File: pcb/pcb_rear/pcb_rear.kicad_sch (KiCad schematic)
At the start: 23 parts, among them J1 MicroLab Input, J2 Pump, J3 DFRobot O2, J4 DFRobot NH3, Q1 T2N7002AK, Q2 T2N7002AK, Q3 T2N7002AK, Q4 T2N7002AK, U1 USEQGSE CO2, U2 USEQGSE CH4, U3 XC9265A331MR-G, U4 XC9265A331MR-G

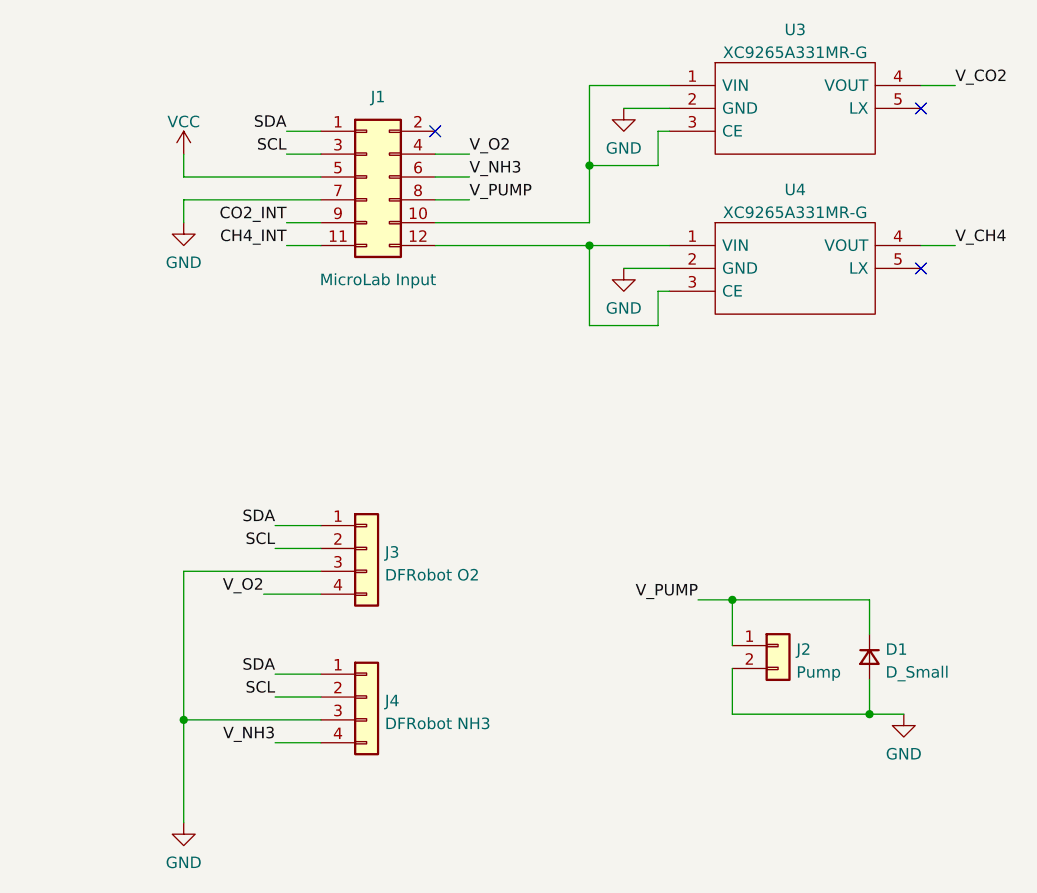
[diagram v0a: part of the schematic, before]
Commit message: front pcb 1st rev
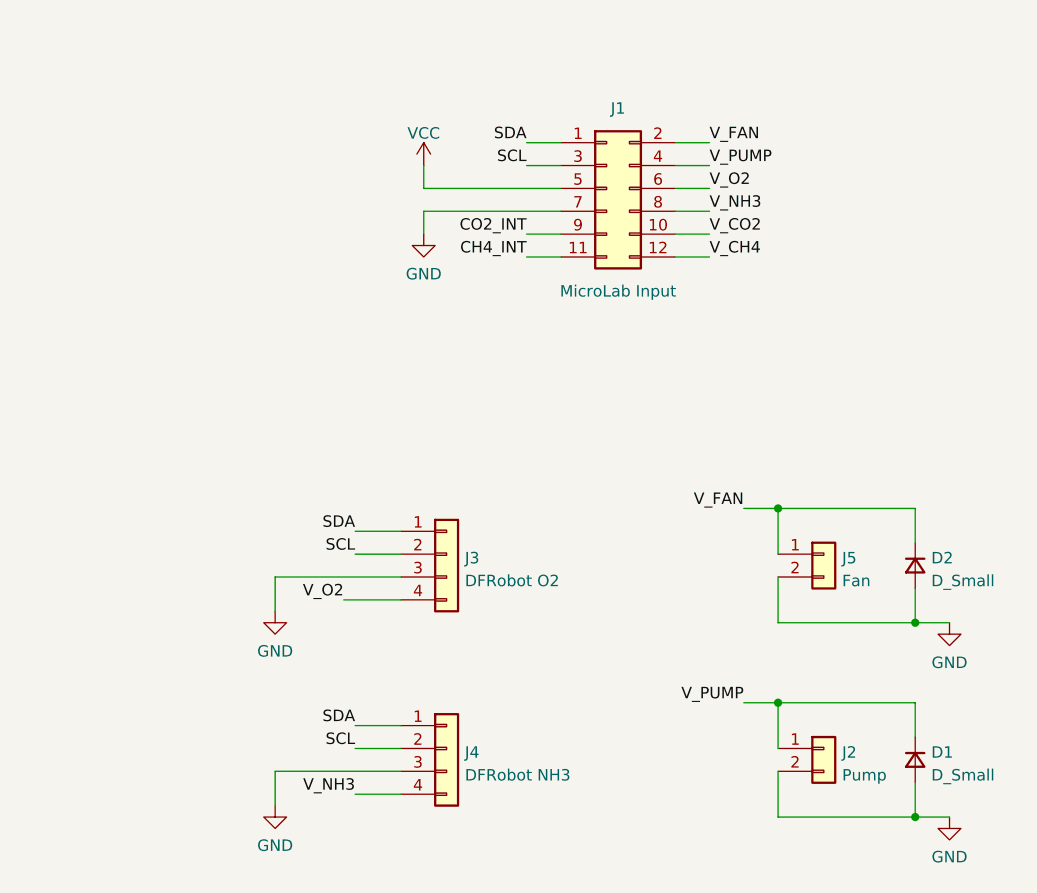
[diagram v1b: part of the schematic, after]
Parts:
- removed U3, U4: XC9265A331MR-G, SamacSys:SOT95P280X130-5N, symbol SamacSys:XC9265A331MR-G
- added D2: D_Small, Diode_SMD:D_0603_1608Metric, symbol Device:D_Small
- added J5: Fan, Connector_PinSocket_2.54mm:PinSocket_1x02_P2.54mm_Vertical, symbol Connector_Generic:Conn_01x02
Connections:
- net GND: now also D2.2 (A), J5.2 (Pin_2)
- net V_CH4: now also J1.12 (Pin_12)
- net V_CO2: now also J1.10 (Pin_10)
- net V_NH3: now also J1.8 (Pin_8); no longer J1.6 (Pin_6)
- net V_O2: now also J1.6 (Pin_6); no longer J1.4 (Pin_4)
- net V_PUMP: now also J1.4 (Pin_4); no longer J1.8 (Pin_8)
- net V_FAN: now reaches J1.2 (Pin_2)
- net V_FAN: now also D2.1 (K), J5.1 (Pin_1)
- no-connect marks 7 -> 4
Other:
- moved on the sheet: D1, J1, J2, J3, J4

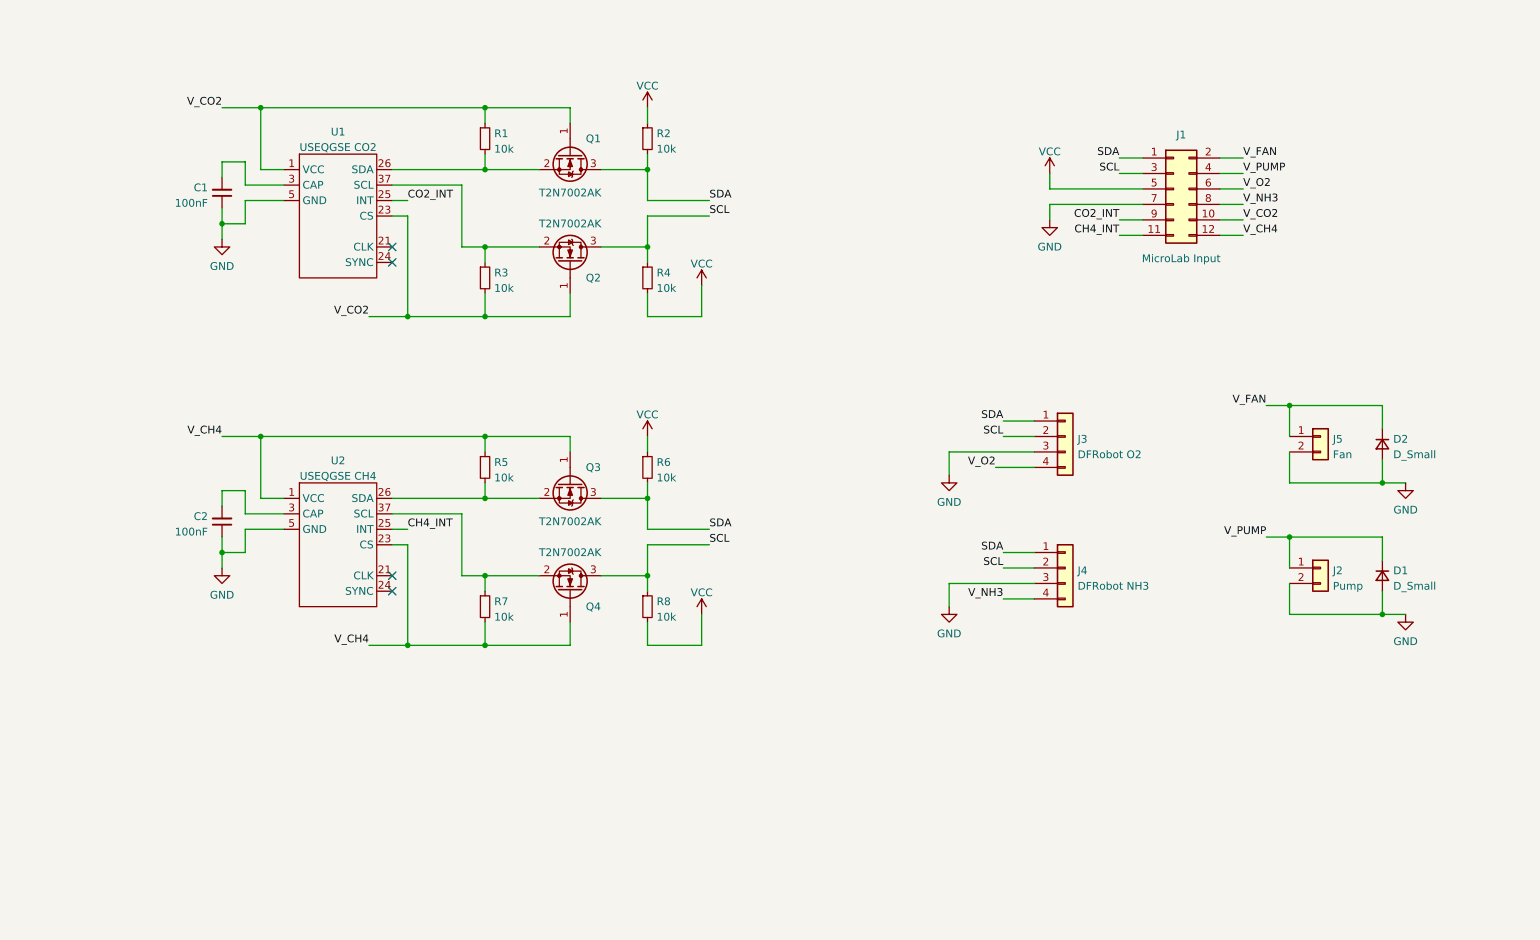
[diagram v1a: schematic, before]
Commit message: fin
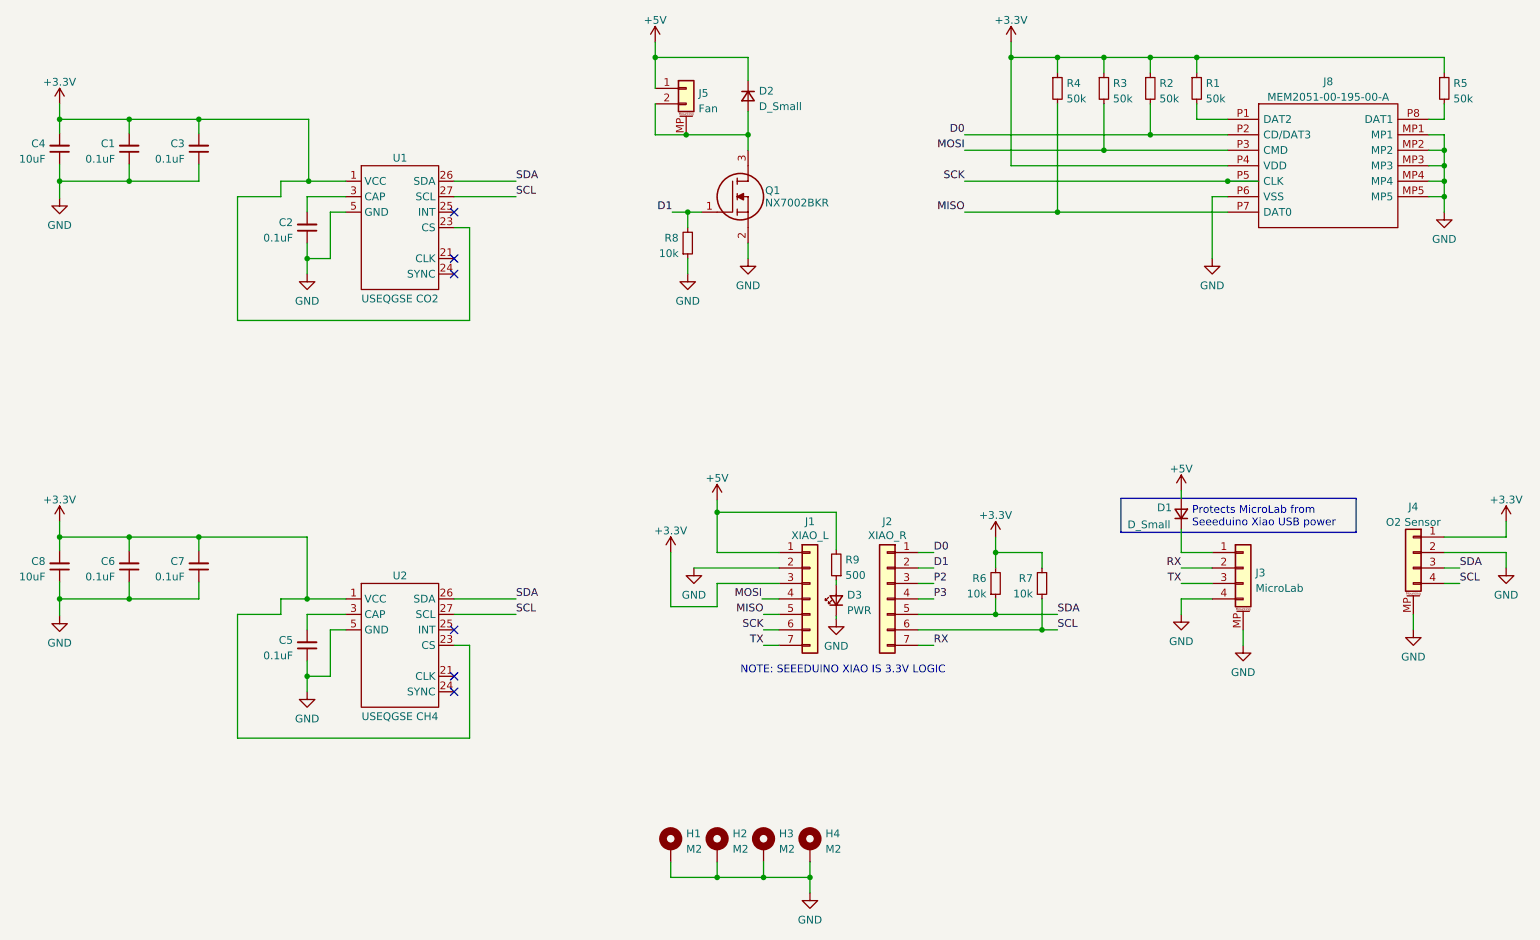
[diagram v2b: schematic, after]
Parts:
- removed C2: 100nF, Capacitor_SMD:C_0603_1608Metric, symbol Device:C_Small
- removed J1: MicroLab Input, Connector_PinSocket_2.54mm:PinSocket_2x06_P2.54mm_Vertical, symbol Connector_Generic:Conn_02x06_Odd_Even
- removed J2: Pump, Connector_PinSocket_2.54mm:PinSocket_1x02_P2.54mm_Vertical, symbol Connector_Generic:Conn_01x02
- removed J3: DFRobot O2, Connector_PinSocket_2.54mm:PinSocket_1x04_P2.54mm_Vertical, symbol Connector_Generic:Conn_01x04
- removed J4: DFRobot NH3, Connector_PinSocket_2.54mm:PinSocket_1x04_P2.54mm_Vertical, symbol Connector_Generic:Conn_01x04
- removed J5: Fan, Connector_PinSocket_2.54mm:PinSocket_1x02_P2.54mm_Vertical, symbol Connector_Generic:Conn_01x02
- removed Q1, Q2, Q3, Q4: T2N7002AK, Package_TO_SOT_SMD:SOT-23, symbol Transistor_FET:BSS138
- added C1, C3, C5, C6, C7: 0.1uF, Capacitor_SMD:C_0402_1005Metric, symbol Device:C_Small
- added C4, C8: 10uF, Capacitor_SMD:C_0402_1005Metric, symbol Device:C_Small
- added D3: PWR, LED_SMD:LED_0402_1005Metric, symbol Device:LED_Small
- added H1, H2, H3, H4: M2, MountingHole:MountingHole_2.2mm_M2_DIN965_Pad, symbol Mechanical:MountingHole_Pad
- added J1: XIAO_L, Connector_PinSocket_2.54mm:PinSocket_1x07_P2.54mm_Vertical, symbol Connector_Generic:Conn_01x07
- added J2: XIAO_R, Connector_PinSocket_2.54mm:PinSocket_1x07_P2.54mm_Vertical, symbol Connector_Generic:Conn_01x07
- added J3: MicroLab, Connector_JST:JST_SH_BM04B-SRSS-TB_1x04-1MP_P1.00mm_Vertical, symbol Connector_Generic_MountingPin:Conn_01x04_MountingPin
- added J4: O2 Sensor, Connector_JST:JST_SH_BM04B-SRSS-TB_1x04-1MP_P1.00mm_Vertical, symbol Connector_Generic_MountingPin:Conn_01x04_MountingPin
- added J5: Fan, Connector_JST:JST_SH_BM02B-SRSS-TB_1x02-1MP_P1.00mm_Vertical, symbol Connector_Generic_MountingPin:Conn_01x02_MountingPin
- added J8: MEM2051-00-195-00-A, SamacSys:MEM20510019500A, symbol Mouser Parts:MEM2051-00-195-00-A
- added Q1: NX7002BKR, Package_TO_SOT_SMD:SOT-23, symbol Mouser Parts:NX7002BKR
- added R9: 500, Resistor_SMD:R_0402_1005Metric, symbol Device:R_Small
- C2: renamed from C1; value 100nF -> 0.1uF; footprint Capacitor_SMD:C_0603_1608Metric -> Capacitor_SMD:C_0402_1005Metric
- D1, D2: footprint Diode_SMD:D_0603_1608Metric -> Diode_SMD:D_SOD-323
- R1, R2, R3, R4, R5: value 10k -> 50k; footprint Resistor_SMD:R_0603_1608Metric -> Resistor_SMD:R_0402_1005Metric
- R6, R7, R8: footprint Resistor_SMD:R_0603_1608Metric -> Resistor_SMD:R_0402_1005Metric
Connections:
- net V_CH4 is gone; now on net +3.3V: R5.1, R7.2, U2.1 (VCC), U2.23 (CS)
- net GND: now also R8.1, C1.1, C3.1, C4.1, C5.1, C6.1, C7.1, C8.1, D3.1 (K), H1.1, H2.1, H3.1, H4.1, J1.2 (Pin_2), J3.4 (Pin_4), J3.MP (MountPin), J4.2 (Pin_2), J4.MP (MountPin), J8.MP1, J8.MP2, J8.MP3, J8.MP4, J8.MP5, J8.P6 (VSS), Q1.2; no longer D1.2 (A), D2.2 (A)
- net SCL: now also R7.1, U1.27 (SCL), U2.27 (SCL), J2.6 (Pin_6), J4.4 (Pin_4); no longer R4.1, R8.1
- net SDA: now also R6.1, U1.26 (SDA), U2.26 (SDA), J2.5 (Pin_5), J4.3 (Pin_3); no longer R2.2, R6.2
- net at R5.2: now also J8.P8 (DAT1); no longer U2.26 (SDA)
- net +3.3V: now reaches R3.1
- net +3.3V: now also R1.1, R2.1, R4.1, R6.2, U1.1 (VCC), U1.23 (CS), C1.2, C3.2, C4.2, C6.2, C7.2, C8.2, J1.3 (Pin_3), J4.1 (Pin_1), J8.P4 (VDD); no longer U1.37 (SCL)
- net at U2.3 (CAP): now also C5.2
- net at R1.2: now also J8.P1 (DAT2); no longer U1.26 (SDA)
- net CH4_INT: no longer names the net of U2.25 (INT)
- net CO2_INT: no longer names the net of U1.25 (INT)
- removed net VCC: R2.1, R4.2, R6.1, R8.2
- removed net V_CO2: R1.1, R3.2, U1.1 (VCC), U1.23 (CS)
- net V_FAN renamed +5V
- net +5V: now also D1.2 (A), J1.1 (Pin_1), J5.1 (Pin_1), R9.2
- net V_PUMP: no longer names the net of D1.1 (K)
- net V_PUMP: now also J3.1 (Pin_1)
- new net: D2.2 (A), J5.2 (Pin_2), J5.MP (MountPin), Q1.3
- new net: D3.2 (A), R9.1
- new net D0: J2.1 (Pin_1), J8.P2 (CD/DAT3), R2.2
- new net D1: J2.2 (Pin_2), Q1.1, R8.2
- new net MISO: J1.5 (Pin_5), J8.P7 (DAT0), R4.2
- new net MOSI: J1.4 (Pin_4), J8.P3 (CMD), R3.2
- new net P2: J2.3 (Pin_3)
- new net P3: J2.4 (Pin_4)
- new net RX: J2.7 (Pin_7), J3.2 (Pin_2)
- new net SCK: J1.6 (Pin_6), J8.P5 (CLK)
- new net TX: J1.7 (Pin_7), J3.3 (Pin_3)
- no-connect marks 4 -> 6
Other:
- note added: "NOTE: SEEEDUINO XIAO IS 3.3V LOGIC"
- note added: "Protects MicroLab from Seeeduino Xiao USB power"
- moved on the sheet: C2, D2, U1
